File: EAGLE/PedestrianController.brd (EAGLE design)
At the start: 57.8 x 85 mm, 16 parts, among them CON1 FTDI, CON2 DS3231, CON3 AC110V, CON4 SIGNAL, IC1 ESP-WROOM-02

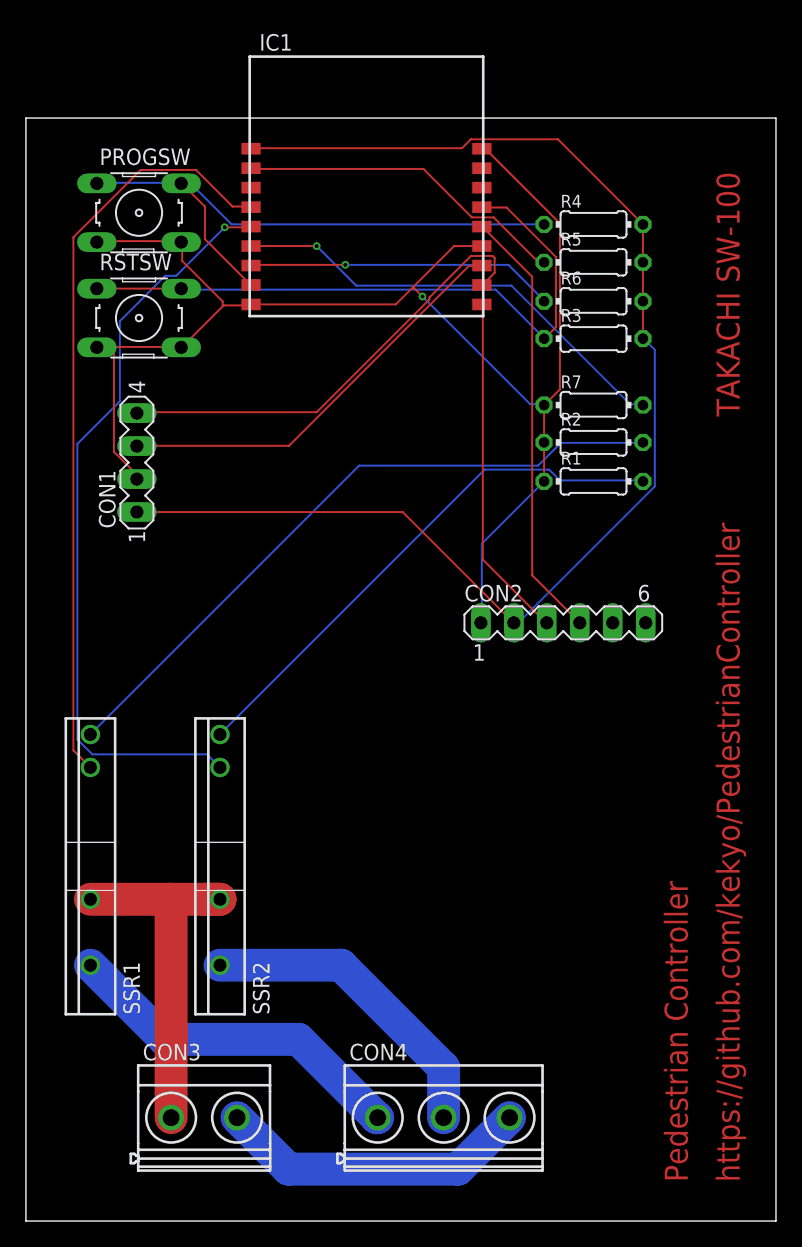
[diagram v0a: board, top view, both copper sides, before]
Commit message: Rerouted with broad rule.
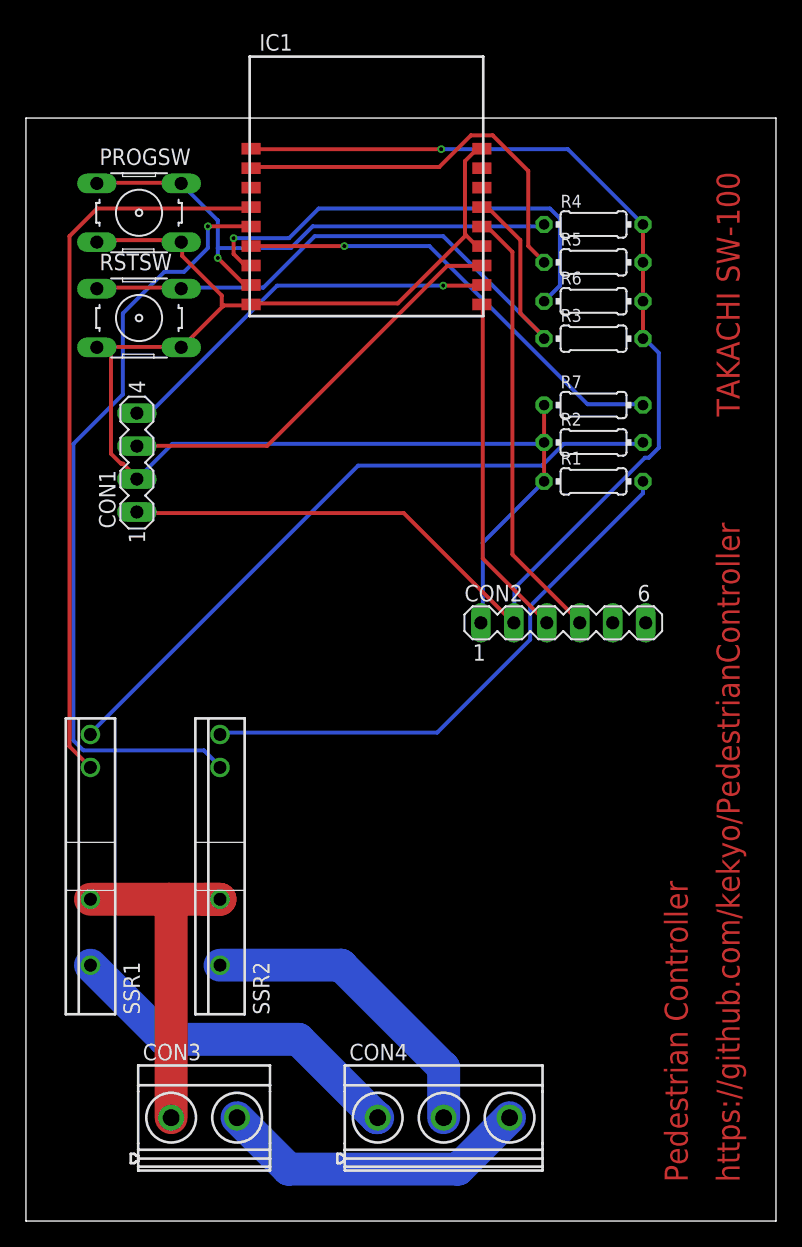
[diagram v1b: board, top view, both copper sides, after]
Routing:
- net N$14: track 23.8 -> 36.2 mm
- net N$13: track 25.6 -> 31.1 mm
- net RXD: track 35.3 -> 30.7 mm, vias 0 -> 1
- net GND: track 113.7 -> 117.7 mm, vias 1 -> 0
- net N$1: track 45.9 -> 42.9 mm, vias 0 -> 1
- net N$9: track 58.4 -> 56.5 mm
- net N$10: track 50.1 -> 52.0 mm
- net N$2: track 58.6 -> 60.3 mm
- net N$4: track 41.5 -> 42.7 mm
- net +3V3: track 101.6 -> 101.3 mm, vias 0 -> 1
